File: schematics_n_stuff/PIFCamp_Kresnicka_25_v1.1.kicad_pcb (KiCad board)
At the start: 2 copper layers, 32.5 x 30 mm, 13 parts, among them J1 Conn_01x01_Pin, U1 ATtiny85-20P, U2 TSOP382xx

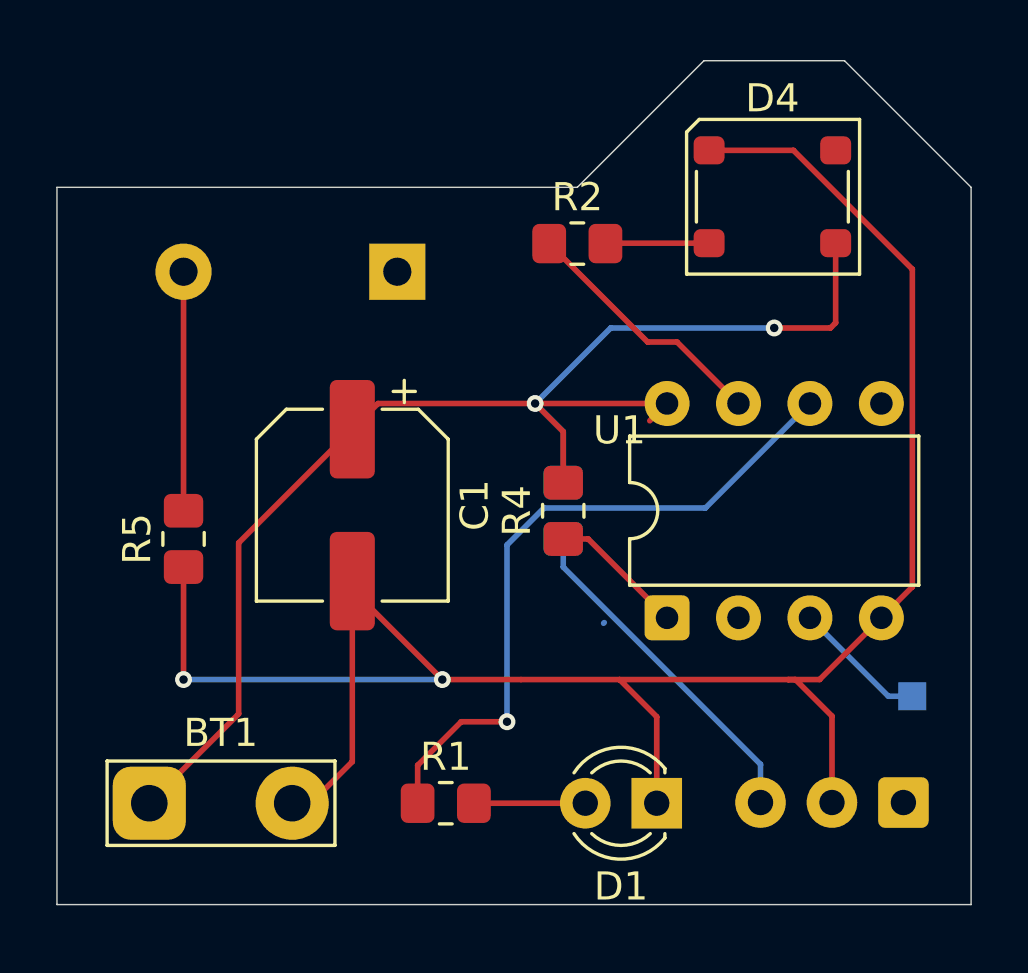
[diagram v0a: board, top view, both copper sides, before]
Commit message: updated pcb
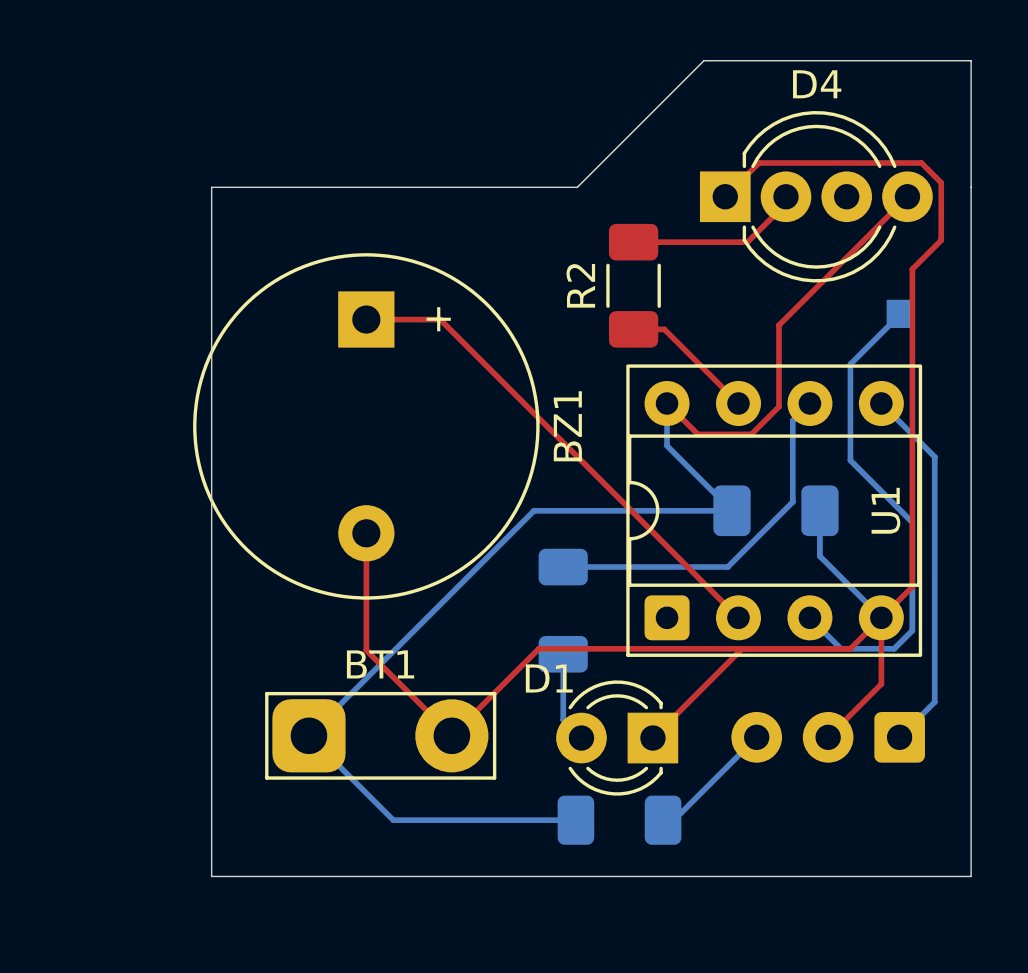
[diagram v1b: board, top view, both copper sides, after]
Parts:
- removed R4: 10K, Resistor_SMD:R_0805_2012Metric_Pad1.20x1.40mm_HandSolder
- removed R5: 22R, Resistor_SMD:R_0805_2012Metric_Pad1.20x1.40mm_HandSolder
- BZ1: moved to F.Cu
- C1: footprint Capacitor_SMD:CP_Elec_6.3x5.8 -> Capacitor_SMD:C_1206_3216Metric_Pad1.33x1.80mm_HandSolder; moved to B.Cu
- D1: footprint LED_THT:LED_D3.0mm_IRBlack -> LED_THT:LED_D3.0mm
- D4: footprint LED_SMD:LED_LiteOn_LTST-E563C_PLCC4_5.0x5.0mm_P3.2mm -> LED_THT:LED_D5.0mm-4_RGB_Wide_Pins
- R1: footprint Resistor_SMD:R_0805_2012Metric_Pad1.20x1.40mm_HandSolder -> Resistor_SMD:R_1206_3216Metric_Pad1.30x1.75mm_HandSolder; moved to B.Cu
- R2, R3: footprint Resistor_SMD:R_0805_2012Metric_Pad1.20x1.40mm_HandSolder -> Resistor_SMD:R_1206_3216Metric_Pad1.30x1.75mm_HandSolder
- U1: footprint Package_DIP:DIP-8_W7.62mm -> Package_DIP:DIP-8_W7.62mm_Socket
- moved C1 15.1 mm to (120.1, 125.5), turned to 0 degrees
- moved J1 13.6 mm to (124.5, 118.5)
- moved R3 11.2 mm to (114.5, 136.5), turned to 180 degrees
- moved R1 8.02 mm to (112.5, 129.1), turned to -90 degrees
- moved BT1 6.16 mm to (103.5, 133.5)
- moved R2 2.50 mm to (115.0, 117.5), turned to 90 degrees
- moved U2 2.32 mm to (124.5, 133.6)
- moved D1 2.32 mm to (115.7, 133.6)
- moved BZ1 2.02 mm to (105.5, 118.7), turned to -90 degrees
- moved D4 1.67 mm to (118.3, 114.3)
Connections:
- BZ1 pad 2: Net-(BZ1--) -> GND
- U1 pad 1: Net-(U1-~{RESET}/PB5) -> unconnected-(U1-~{RESET}/PB5-Pad1)
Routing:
- net Net-(BZ1-+): track 0.00 -> 17.6 mm
- net Net-(U1-AREF/PB0): track 0.00 -> 13.2 mm
- net Net-(J1-Pin_1): track 4.79 -> 17.3 mm
- net Net-(U1-PB1): track 24.3 -> 12.9 mm, vias 1 -> 0
- net /VCC: track 62.4 -> 52.6 mm, vias 2 -> 0
- net Net-(BZ1--): track 8.50 -> 0.00 mm
- net GND: track 75.8 -> 68.4 mm, vias 2 -> 0
- net Net-(U1-~{RESET}/PB5): track 5.69 -> 0.00 mm
- net Net-(U1-PB2): track 9.08 -> 4.82 mm
- net Net-(D4-DIN): track 3.69 -> 6.23 mm
- net unconnected-(U1-~{RESET}/PB5-Pad1): track 0.00 -> 0.84 mm
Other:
- board size 32.5 x 30 mm -> 27 x 29 mm
